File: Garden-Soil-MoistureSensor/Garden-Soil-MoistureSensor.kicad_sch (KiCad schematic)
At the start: 6 parts, among them J1 Conn_01x15, J2 Conn_01x15, J3 Screw_Terminal_01x02, U1 1043

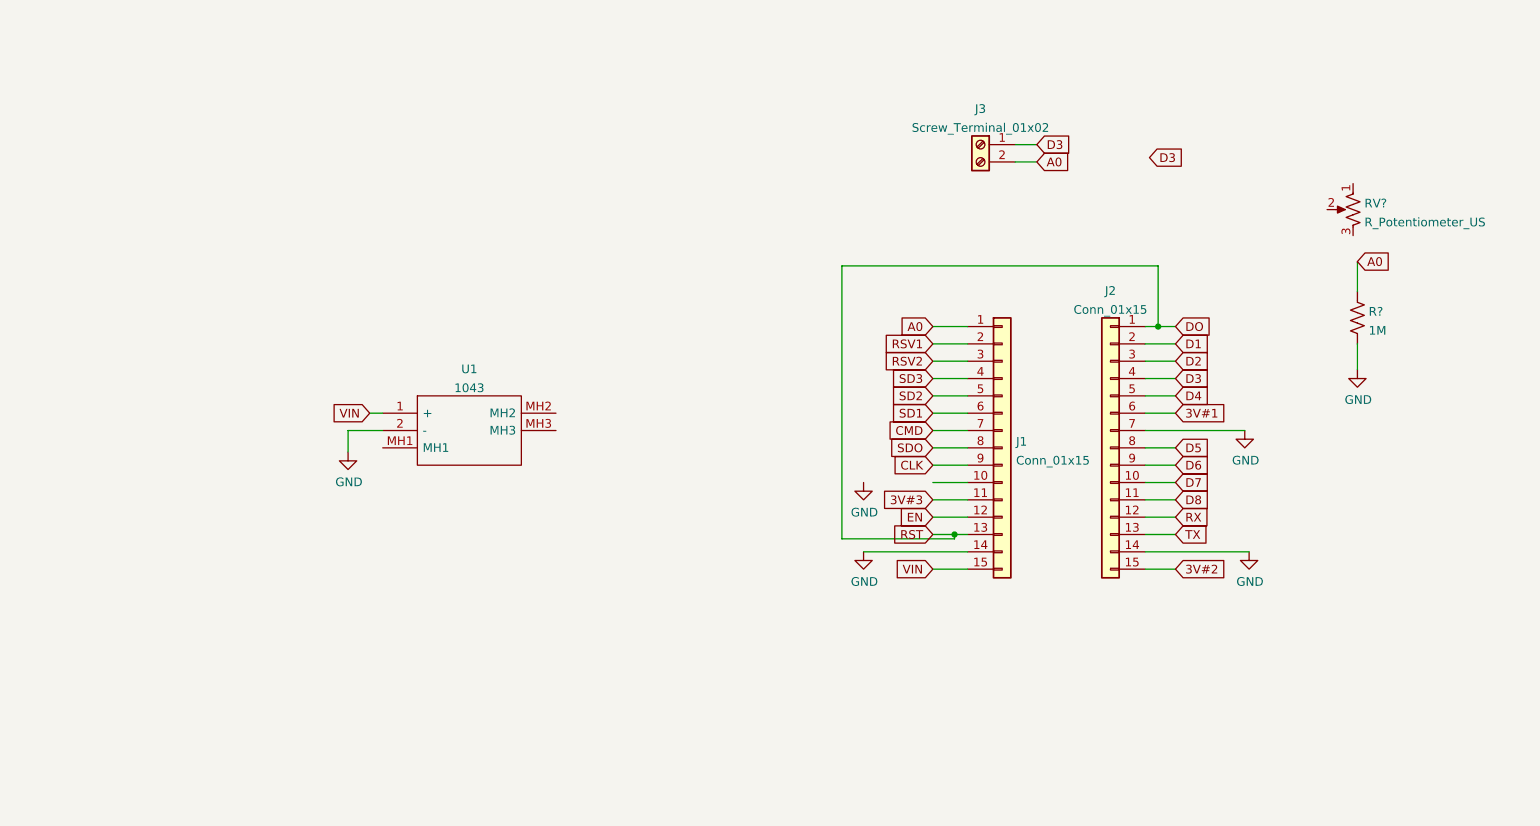
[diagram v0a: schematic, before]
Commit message: wip on adding the MUXes.
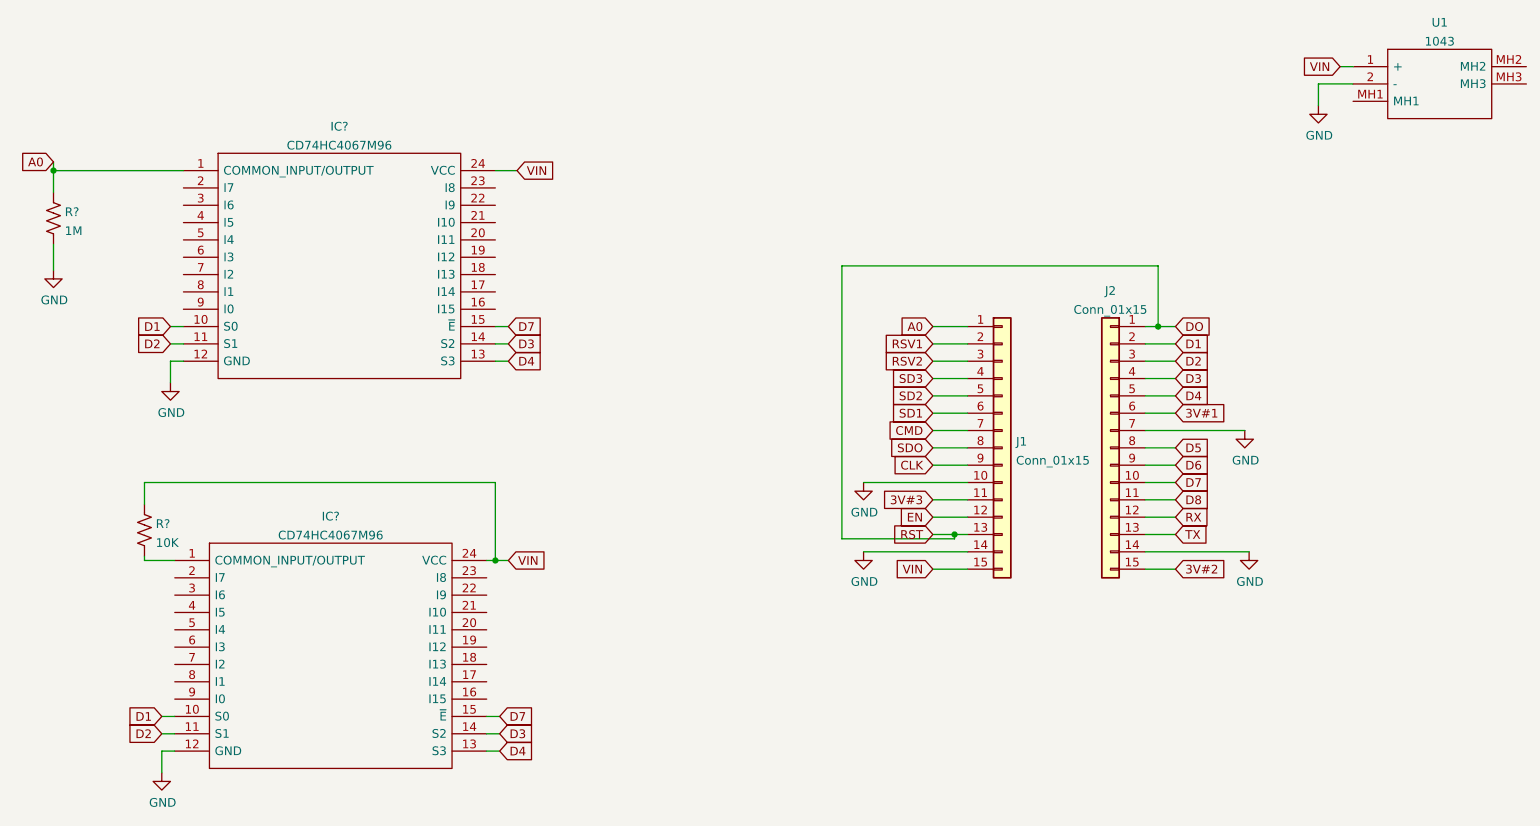
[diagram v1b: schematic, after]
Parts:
- removed J3: Screw_Terminal_01x02, TerminalBlock_Phoenix:TerminalBlock_Phoenix_MKDS-1,5-2_1x02_P5.00mm_Horizontal, symbol Connector:Screw_Terminal_01x02
- removed RV?: R_Potentiometer_US, symbol Device:R_Potentiometer_US
- added IC? (x2): CD74HC4067M96, SOIC127P1030X265-24N, symbol Samac_Sys:CD74HC4067M96
- added R?: 10K, symbol Device:R_US
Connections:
- net A0: now also IC?.1 (COMMON_INPUT/OUTPUT)
- net D1: now also IC?.10 (S0), IC?.10 (S0)
- net D2: now also IC?.11 (S1), IC?.11 (S1)
- net D3: now also IC?.14 (S2), IC?.14 (S2)
- net D4: now also IC?.13 (S3), IC?.13 (S3)
- net D7: now also IC?.15 (~{E}), IC?.15 (~{E})
- net GND: now also J1.10 (Pin_10), IC?.12 (GND), IC?.12 (GND)
- net VIN: now also IC?.24 (VCC), IC?.24 (VCC), R?.1
- new net: IC?.1 (COMMON_INPUT/OUTPUT), R?.2
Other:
- moved on the sheet: R?, U1
